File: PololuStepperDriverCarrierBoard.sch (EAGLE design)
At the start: 42 parts, among them J1 MS1, J10 Y Stepper, J11 Interface, J12 MS1, J13 MS2, J14 A4988BREAKOUT, J15 MS3, J16 Z Stepper, J17 MS1, J18 24V Input, J19 MS2, J2 MS2, J20 A4988BREAKOUT, J21 MS3, J22 E1 Stepper, J23 MS1, J24 MS2, J25 A4988BREAKOUT, J26 MS3, J27 E2 Stepper, J3 A4988BREAKOUT, J4 MS3, J5 X Stepper, J6 MS1, J7 MS2, J8 A4988BREAKOUT, J9 MS3

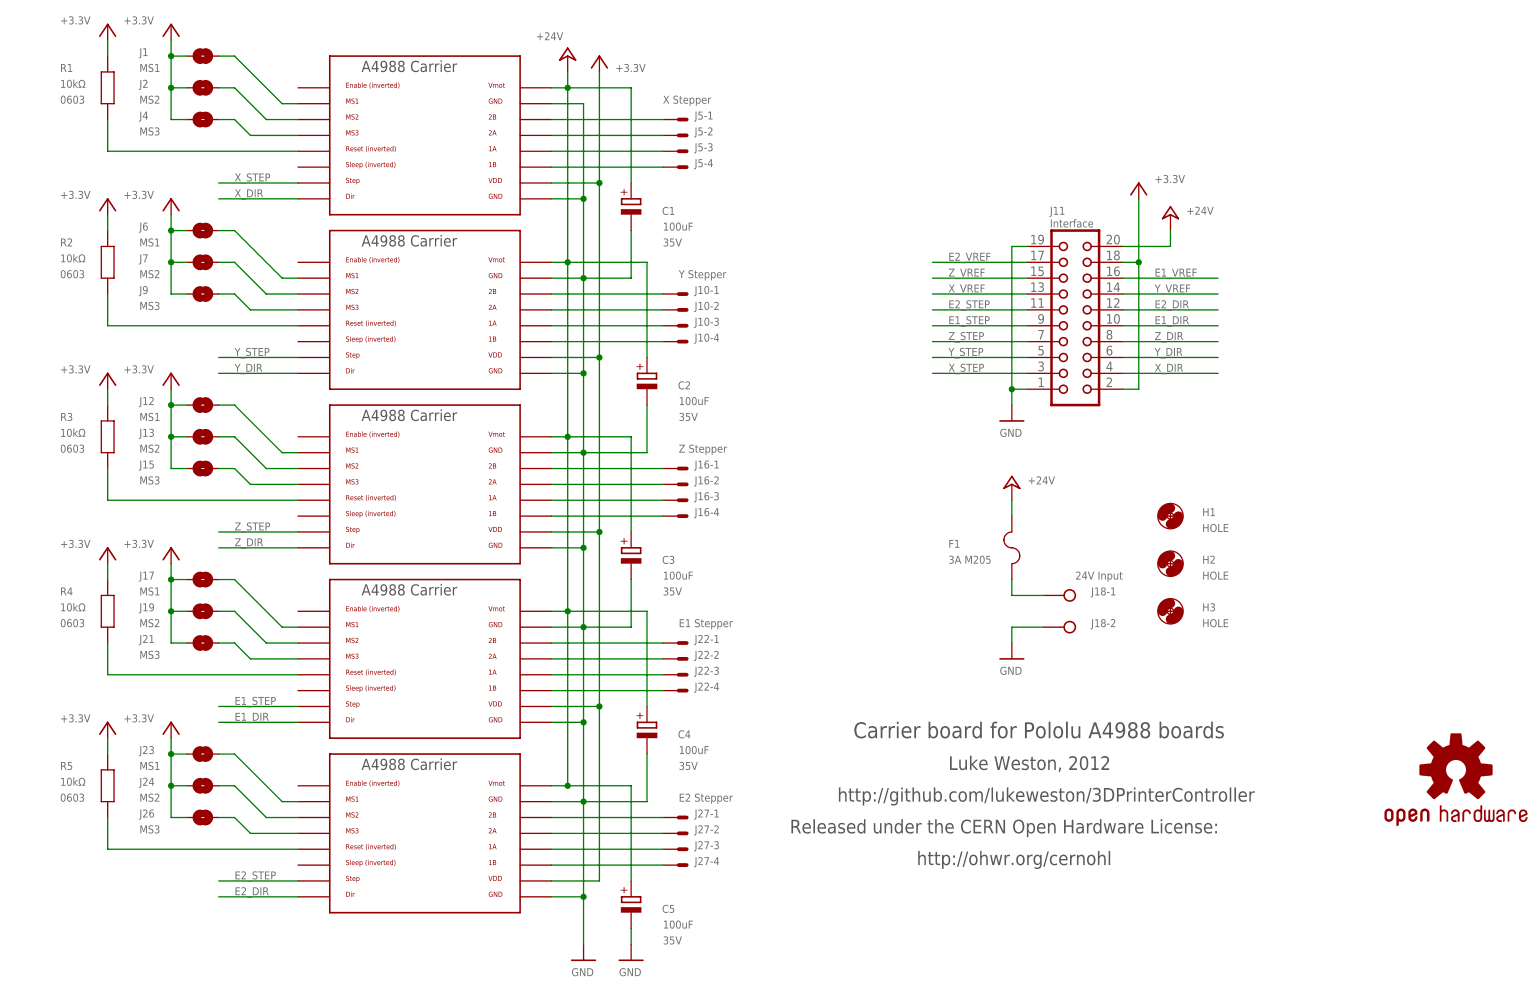
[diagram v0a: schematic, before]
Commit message: foo
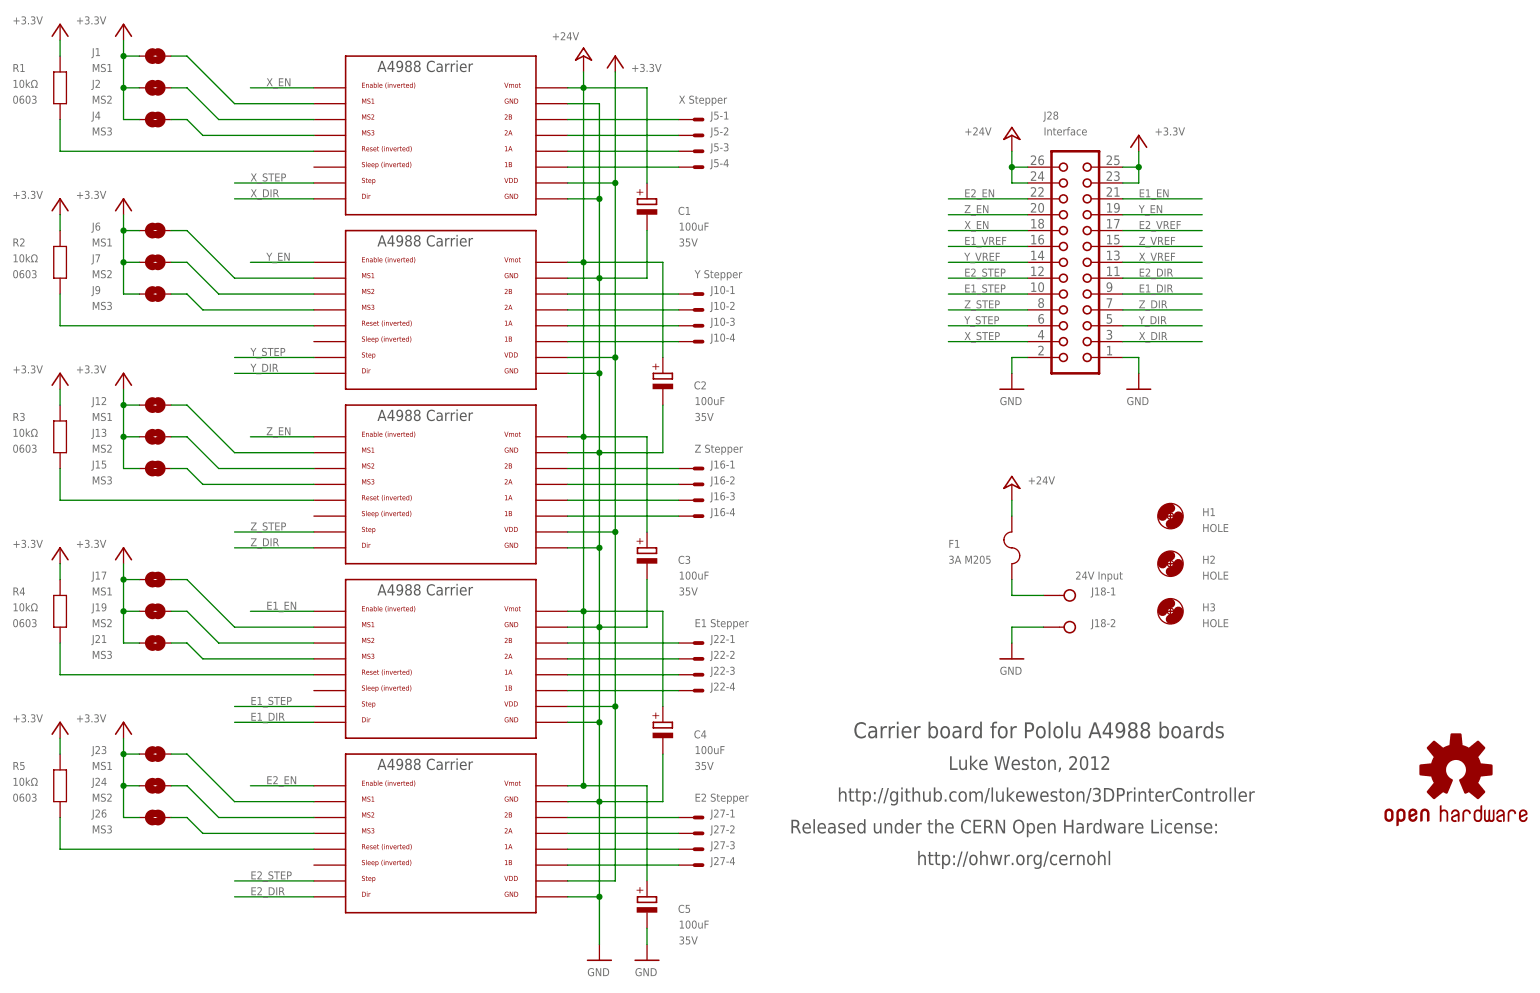
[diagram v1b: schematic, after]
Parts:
- removed J11: Interface, con-harting:CON20L
- added J28: Interface, con-harting:CON26L
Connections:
- new net E1_EN: J20.EN, J28.21
- new net E2_EN: J25.EN, J28.22
- new net X_EN: J28.18, J3.EN
- new net Y_EN: J28.19, J8.EN
- new net Z_EN: J14.EN, J28.20
- net +24V: now also J28.24, J28.26; no longer J11.20
- net +3V3: now also J28.23, J28.25; no longer J11.18, J11.2
- net E1_DIR: now also J28.9; no longer J11.10
- net E1_STEP: now also J28.10; no longer J11.9
- net E1_VREF: now also J28.16; no longer J11.16
- net E2_DIR: now also J28.11; no longer J11.12
- net E2_STEP: now also J28.12; no longer J11.11
- net E2_VREF: now also J28.17; no longer J11.17
- net GND: now also J28.1, J28.2; no longer J11.1, J11.19
- net X_DIR: now also J28.3; no longer J11.4
- net X_STEP: now also J28.4; no longer J11.3
- net X_VREF: now also J28.13; no longer J11.13
- net Y_DIR: now also J28.5; no longer J11.6
- net Y_STEP: now also J28.6; no longer J11.5
- net Y_VREF: now also J28.14; no longer J11.14
- net Z_DIR: now also J28.7; no longer J11.8
- net Z_STEP: now also J28.8; no longer J11.7
- net Z_VREF: now also J28.15; no longer J11.15
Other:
- moved on the sheet: C1, C2, C3, C4, C5, J1, J10-1, J10-2, J10-3, J10-4, J12, J13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
